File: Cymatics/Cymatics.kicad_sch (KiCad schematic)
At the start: 75 parts, among them IC1 LMV358IDR, IC2 MAX7403CSA+, IC3 LMV358IDR, IC4 LMV358IDR, IC5 MAX7403CSA+, J1 Screw_Terminal_01x03, J10 Screw_Terminal_01x04, J11 Screw_Terminal_01x05, J12 Screw_Terminal_01x02, J13 Screw_Terminal_01x02, J14 RCU-0C, J15 Screw_Terminal_01x02, J16 Screw_Terminal_01x03, J17 Screw_Terminal_01x02, J18 Screw_Terminal_01x06, J19 RCU-0C, J2 Screw_Terminal_01x02, J20 RCU-0C, J21 RCU-0C, J22 RCU-0C, J23 RCU-0C, J24 RCU-0C, J3 Screw_Terminal_01x03, J4 Screw_Terminal_01x03, J5 Screw_Terminal_01x02, J6 Conn_01x16_Socket, J7 Conn_01x12_Socket, J8 Screw_Terminal_01x04, J9 Screw_Terminal_01x02, U1 SN74AHCT125DR, U2 MAX7480ESA+

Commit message: Order for March PCB
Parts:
- C1, C10, C11, C15, C2, C6, C7, C8: In Stock 02-26-25 (none) -> 10; To Order 02-26-25 (none) -> 20
- C12, C13, C16, C18, C3, C4, C9: In Stock 02-26-25 (none) -> 8; To Order 02-26-25 (none) -> 20
- C14, C5, R10, R11, R14, R22, R23, R9: In Stock 02-26-25 (none) -> 5; To Order 02-26-25 (none) -> 10
- C17, J18, J6, J7, RN2, SD1, U1, U2: In Stock 02-26-25 (none) -> 0; To Order 02-26-25 (none) -> 3
- C19: In Stock 02-26-25 (none) -> 9; To Order 02-26-25 (none) -> 0
- IC1, IC3, IC4: In Stock 02-26-25 (none) -> 3; To Order 02-26-25 (none) -> 6
- IC2, IC5: In Stock 02-26-25 (none) -> 0; To Order 02-26-25 (none) -> 6
- J1, J16, J3, J4: In Stock 02-26-25 (none) -> 3; To Order 02-26-25 (none) -> 9
- J10, J11, J8: In Stock 02-26-25 (none) -> 1; To Order 02-26-25 (none) -> 2
- J12, J13, J15, J17, J2, J5, J9: In Stock 02-26-25 (none) -> 4; To Order 02-26-25 (none) -> 11
- J14, J19, J20, J21, J22, J23, J24: In Stock 02-26-25 (none) -> 3; To Order 02-26-25 (none) -> 18
- R1, R12, R13, R16, R17, R2, R20, R21, R24, R25, R3, R4, R7, R8: In Stock 02-26-25 (none) -> 4; To Order 02-26-25 (none) -> 50
- R5, R6: In Stock 02-26-25 (none) -> 6; To Order 02-26-25 (none) -> 0
- RN1: footprint CAY16:RESCAF80P320X160X60-8N -> CAY16-473:RESCAF80P320X160X60-8N; In Stock 02-26-25 (none) -> 0; To Order 02-26-25 (none) -> 3

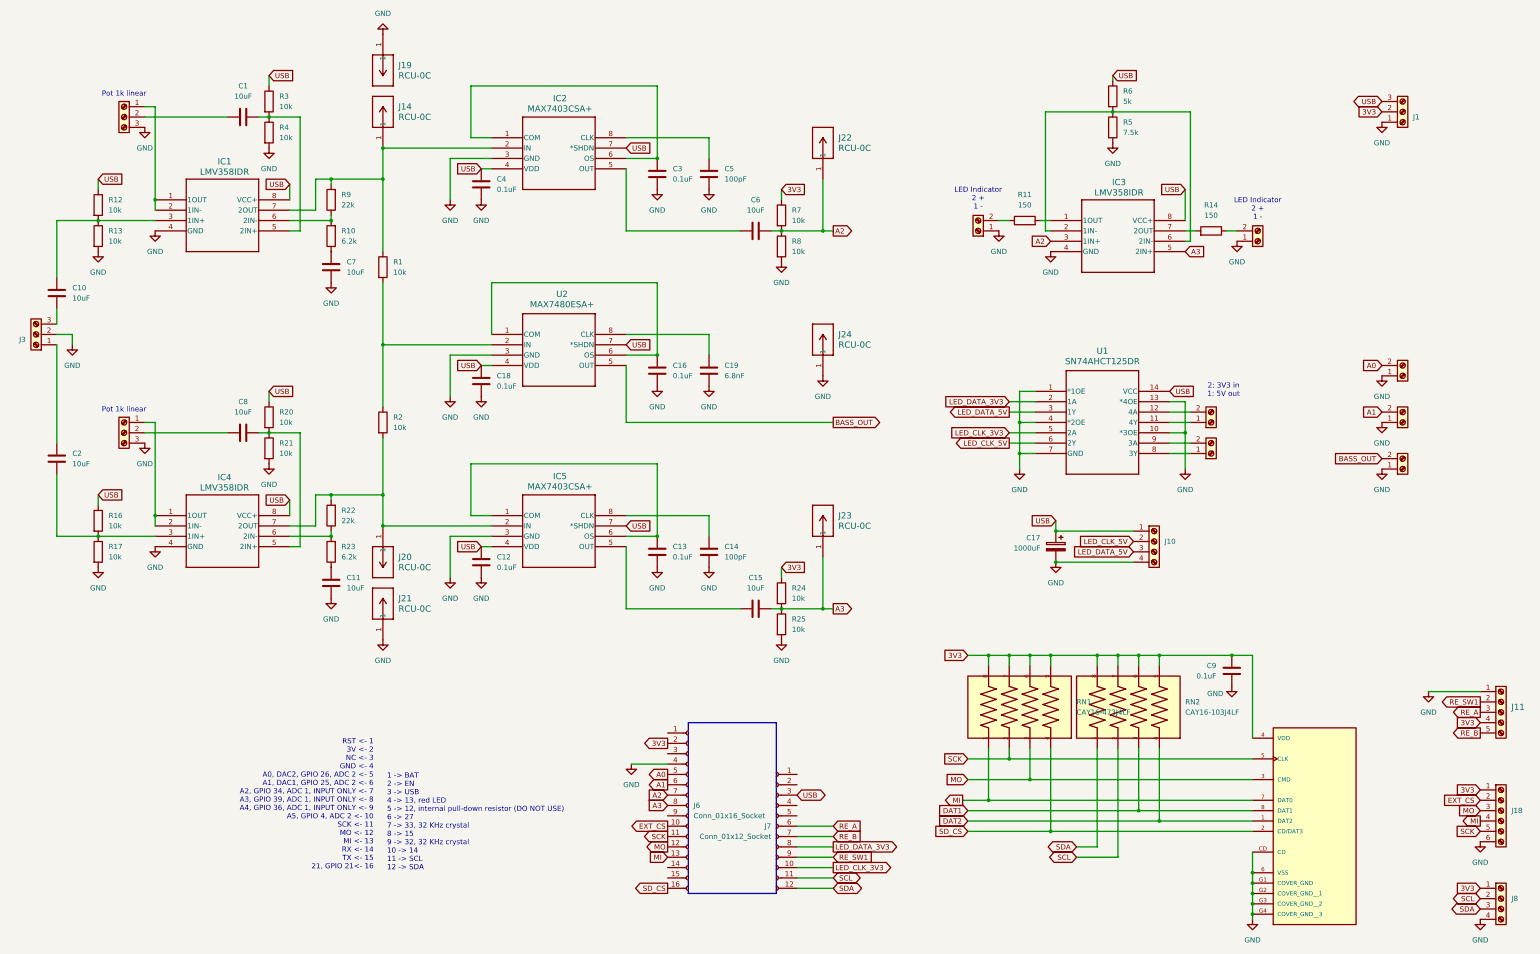
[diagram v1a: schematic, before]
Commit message: All changes up through Week 9, including making the step file
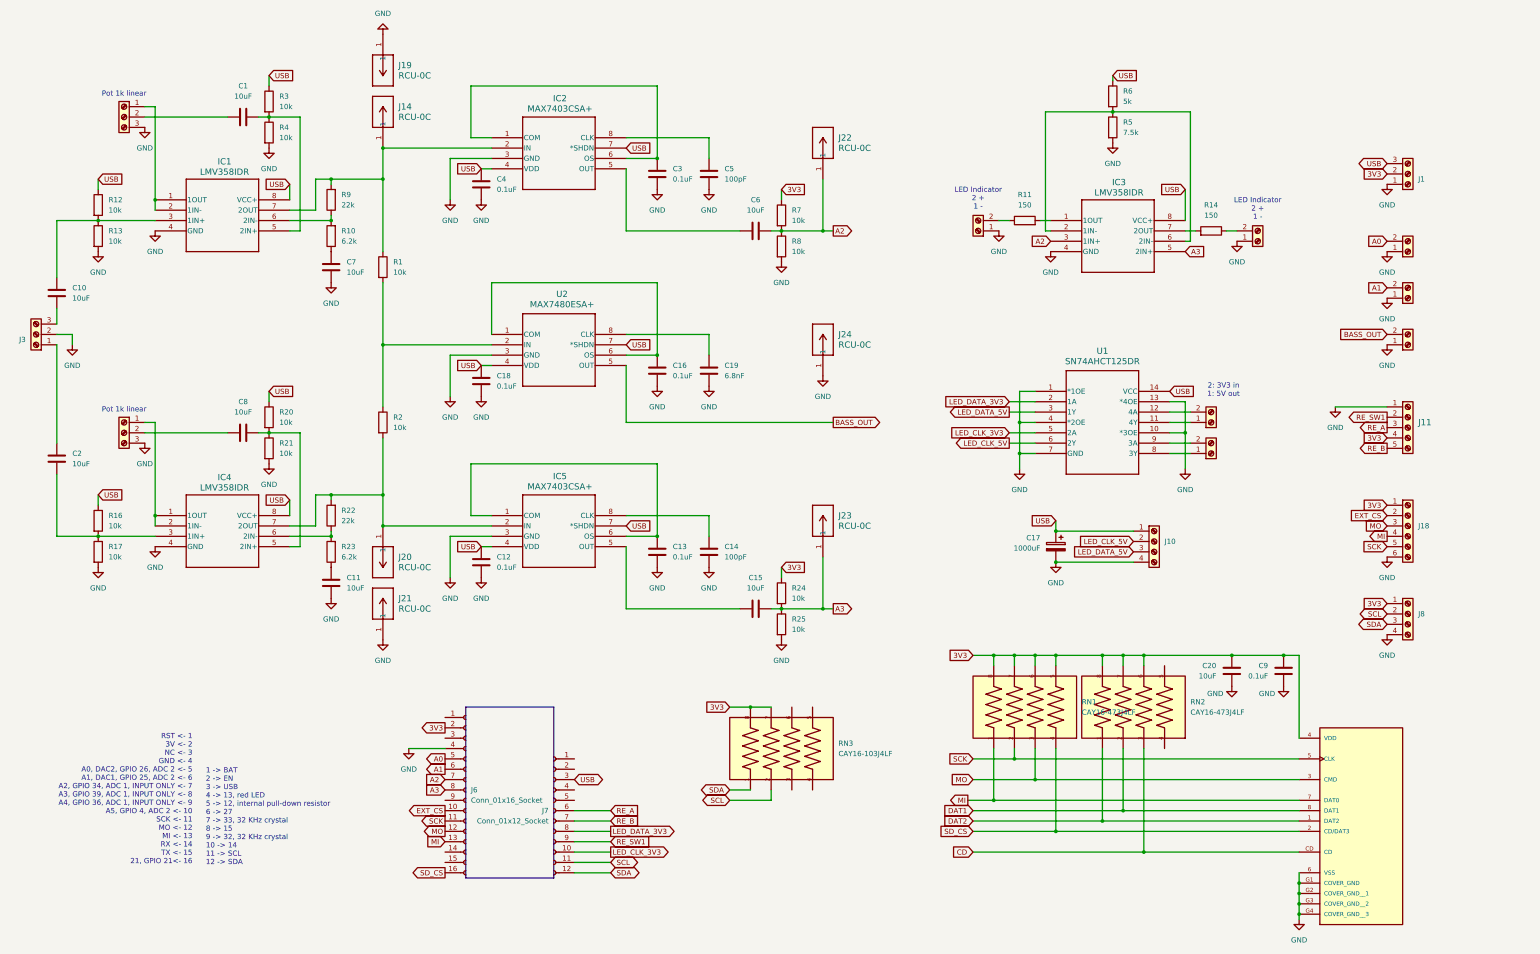
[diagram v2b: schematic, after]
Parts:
- removed RN2: CAY16-103J4LF, CAY16-103:RESCAF80P320X160X60-8N, symbol CAY16-103:CAY16-103J4LF
- added C20: 10uF, Capacitor_SMD:C_0805_2012Metric, symbol Device:C
- added RN2: CAY16-473J4LF, CAY16-473:RESCAF80P320X160X60-8N, symbol CAY16:CAY16-473J4LF
- added RN3: CAY16-103J4LF, CAY16-103:RESCAF80P320X160X60-8N, symbol CAY16-103:CAY16-103J4LF
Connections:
- net 3V3: now also C20.1, RN2.6, RN2.7, RN2.8, RN3.7, RN3.8
- net DAT1: now also RN2.2
- net DAT2: now also RN2.1
- net GND: now also C20.2; no longer SD1.CD
- net SCL: now also RN3.2
- net SDA: now also RN3.1
- new net CD: RN2.3, SD1.CD
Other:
- note added: "1 -> BAT 2 -> EN 3 -> USB 4 -> 13, red LED 5 -> 12, internal pull-down resistor 6 -> 27 7 -> 33, 32 KHz crystal 8 -> 15 9 -> 32, 32 KHz crystal 10 -> 14 11 -> SCL 12 -> SDA"
- note removed: "1 -> BAT 2 -> EN 3 -> USB 4 -> 13, red LED 5 -> 12, internal pull-down resistor (DO NOT USE) 6 -> 27 7 -> 33, 32 KHz crystal 8 -> 15 9 -> 32, 32 KHz crystal 10 -> 14 11 -> SCL 12 -> SDA"
- moved on the sheet: C9, J1, J11, J18, J6, J7, J8, RN1
